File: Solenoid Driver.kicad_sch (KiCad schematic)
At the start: 5 parts, among them U1 DRV8837

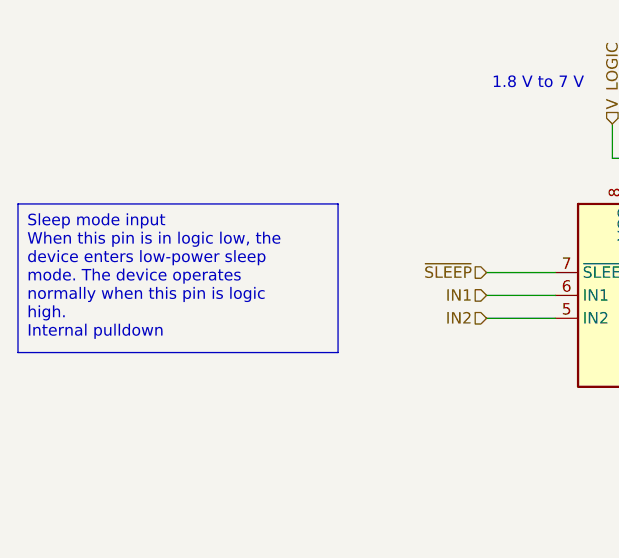
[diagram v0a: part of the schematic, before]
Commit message: Progress?
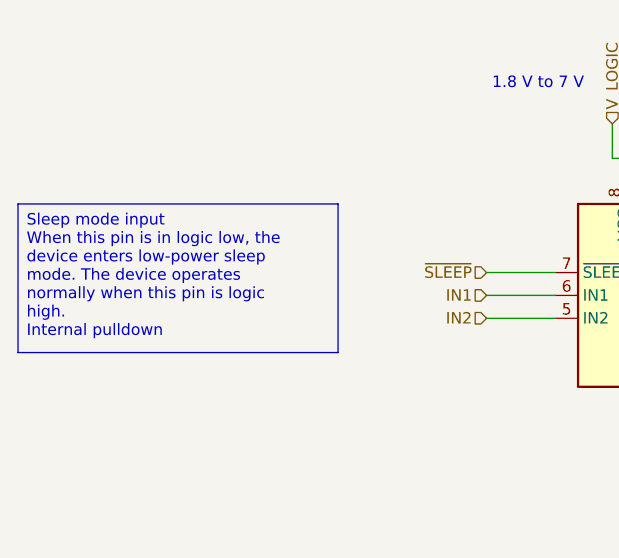
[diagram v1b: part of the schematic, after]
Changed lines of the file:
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@@
 (kicad_sch
-	(version 20231120)
+	(version 20250114)
 	(generator "eeschema")
-	(generator_version "8.0")
+	(generator_version "9.0")
 	(paper "A4")
+	(rectangle
+		(start 224.79 115.57)
+		(end 280.67 161.29)
+		(stroke
+			(width 0)
+			(type dash)
+		)
+		(fill
+			(type none)
+		)
+	)
+	(text "Motor output"
+		(exclude_from_sim no)
+		(at 175.26 99.06 0)
+		(effects
+			(font
+				(size 1.27 1.27)
+			)
+		)
+	)
+	(text "0 V to 11 V"
+		(exclude_from_sim no)
+		(at 161.29 75.565 0)
+		(effects
+			(font
+				(size 1.27 1.27)
+			)
+		)
+	)
+	(text "Decoupling"
+		(exclude_from_sim no)
+		(at 253.365 118.745 0)
+		(effects
+			(font
+				(size 1.905 1.905)
+			)
+		)
+	)
+	(text "1.8 V to 7 V"
+		(exclude_from_sim no)
+		(at 140.335 75.565 0)
+		(effects
+			(font
+				(size 1.27 1.27)
+			)
+		)
+	)
+	(text_box "Sleep mode input\nWhen this pin is in logic low, the device enters low-power sleep mode. The device operates\nnormally when this pin is logic high. \nInternal pulldown"
+		(exclude_from_sim no)
+		(at 82.55 88.9 0)
+		(size 35.56 16.51)
+		(margins 0.9525 0.9525 0.9525 0.9525)
+		(stroke
+			(width 0)
+			(type default)
+		)
+		(fill
+			(type none)
+		)
+		(effects
+			(font
+				(size 1.27 1.27)
+			)
+			(justify left top)
+		)
+	)
 	(junction
 		(at 257.81 135.89)
@@
 		)
 	)
-	(rectangle
-		(start 224.79 115.57)
-		(end 280.67 161.29)
-		(stroke
-			(width 0)
-			(type dash)
-		)
-		(fill
-			(type none)
-		)
-	)
-	(text_box "Sleep mode input\nWhen this pin is in logic low, the device enters low-power sleep mode. The device operates\nnormally when this pin is logic high. \nInternal pulldown"
-		(exclude_from_sim no)
-		(at 82.55 88.9 0)
-		(size 35.56 16.51)
-		(stroke
-			(width 0)
-			(type default)
-		)
-		(fill
-			(type none)
-		)
-		(effects
-			(font
-				(size 1.27 1.27)
-			)
-			(justify left top)
-		)
-	)
-	(text "Motor output"
-		(exclude_from_sim no)
-		(at 175.26 99.06 0)
-		(effects
-			(font
-				(size 1.27 1.27)
-			)
-		)
-	)
-	(text "0 V to 11 V"
-		(exclude_from_sim no)
-		(at 161.29 75.565 0)
-		(effects
-			(font
-				(size 1.27 1.27)
-			)
-		)
-	)
-	(text "Decoupling"
-		(exclude_from_sim no)
-		(at 253.365 118.745 0)
-		(effects
-			(font
-				(size 1.905 1.905)
-			)
-		)
-	)
-	(text "1.8 V to 7 V"
-		(exclude_from_sim no)
-		(at 140.335 75.565 0)
-		(effects
-			(font
-				(size 1.27 1.27)
-			)
-		)
-	)
 	(hierarchical_label "0V"
 		(shape input)
 		(at 257.81 154.94 270)
-		(fields_autoplaced yes)
 		(effects
 			(font
@@
 		(shape input)
 		(at 148.59 80.01 90)
-		(fields_autoplaced yes)
 		(effects
 			(font
@@
 		(shape input)
 		(at 257.81 132.08 90)
-		(fields_autoplaced yes)
 		(effects
 			(font
@@
 		(shape input)
 		(at 152.4 114.3 270)
-		(fields_autoplaced yes)
 		(effects
 			(font
@@
 		(shape input)
 		(at 134.62 96.52 180)
-		(fields_autoplaced yes)
 		(effects
 			(font
@@
 		(shape input)
 		(at 229.87 135.89 90)
-		(fields_autoplaced yes)
 		(effects
 			(font
@@
 		(shape input)
 		(at 134.62 99.06 180)
-		(fields_autoplaced yes)
 		(effects
 			(font
@@
 		(shape input)
 		(at 229.87 151.13 270)
-		(fields_autoplaced yes)
 		(effects
 			(font
@@
 		(shape input)
 		(at 134.62 101.6 180)
-		(fields_autoplaced yes)
 		(effects
 			(font
@@
 		(shape input)
 		(at 153.67 80.01 90)
-		(fields_autoplaced yes)
 		(effects
 			(font
@@
 		(shape input)
 		(at 170.18 91.44 0)
-		(fields_autoplaced yes)
 		(effects
 			(font
@@
 		(shape input)
 		(at 170.18 106.68 0)
-		(fields_autoplaced yes)
-		(effects
-			(font
+		(effects
+			(font
